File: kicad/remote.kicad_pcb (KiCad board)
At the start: 2 copper layers, 62 parts, among them J1 Conn_01x03, J10 Conn_01x03, J11 Conn_01x03, J12 Conn_01x02, J13 Conn_01x04, J14 Conn_01x04, J2 Conn_01x02, J3 Conn_01x07, J4 Conn_01x03, J5 Conn_01x03, J6 Conn_01x02, J7 Conn_01x03, J8 Conn_01x08, J9 Conn_01x08, SW1 SW_SPDT_MSM, SW10 SW_Push, SW11 SW_DP3T, SW2 SW_SPDT_MSM, SW3 SW_SPDT_MSM, SW4 SW_SPDT_MSM, SW5 SW_Push, SW6 SW_Push, SW7 SW_Push, SW8 SW_Push, SW9 SW_Push, U1 74LS165, U2 74LS165, U3 Arduino_Nano_v3.x, U4 AP1117, U5 nRF24L01+, U6 OLED_7pin_4SPI, U7 COM-09032, U8 COM-09032

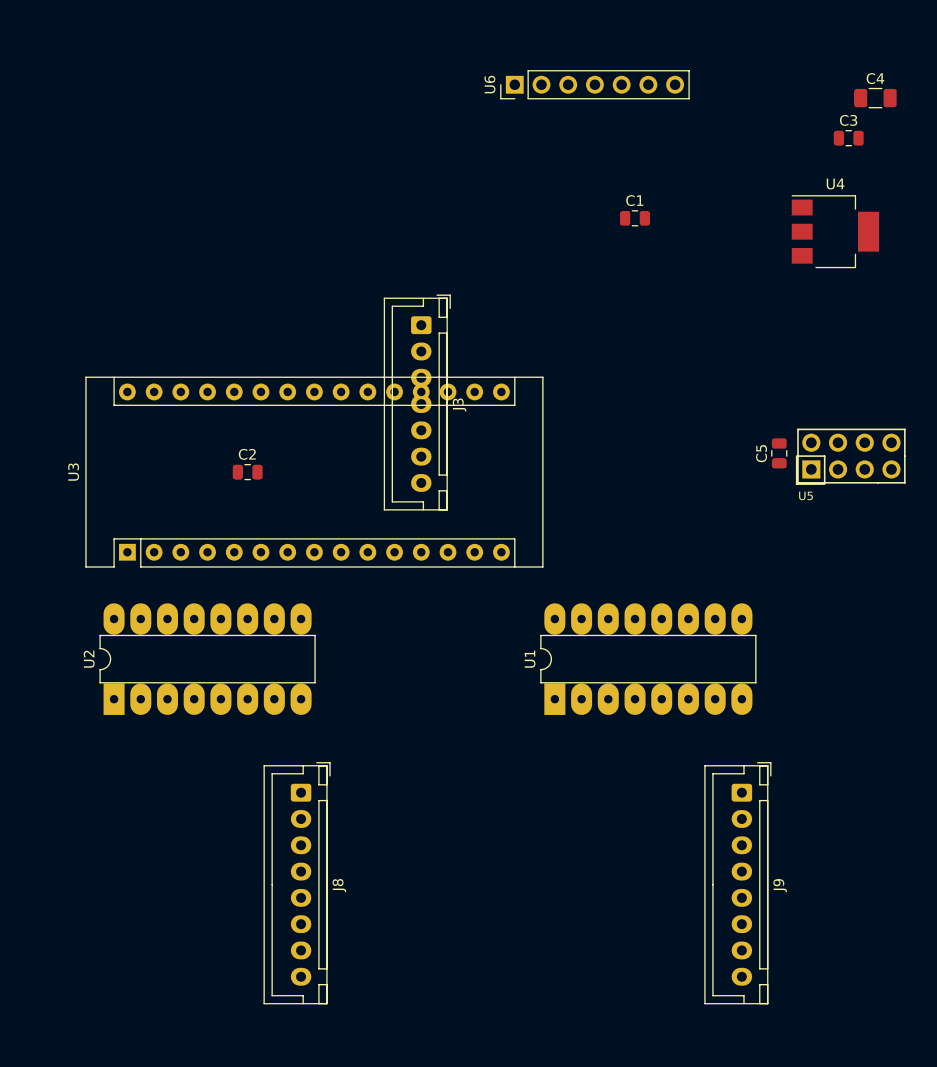
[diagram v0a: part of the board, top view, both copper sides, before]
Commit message: Work on layout.
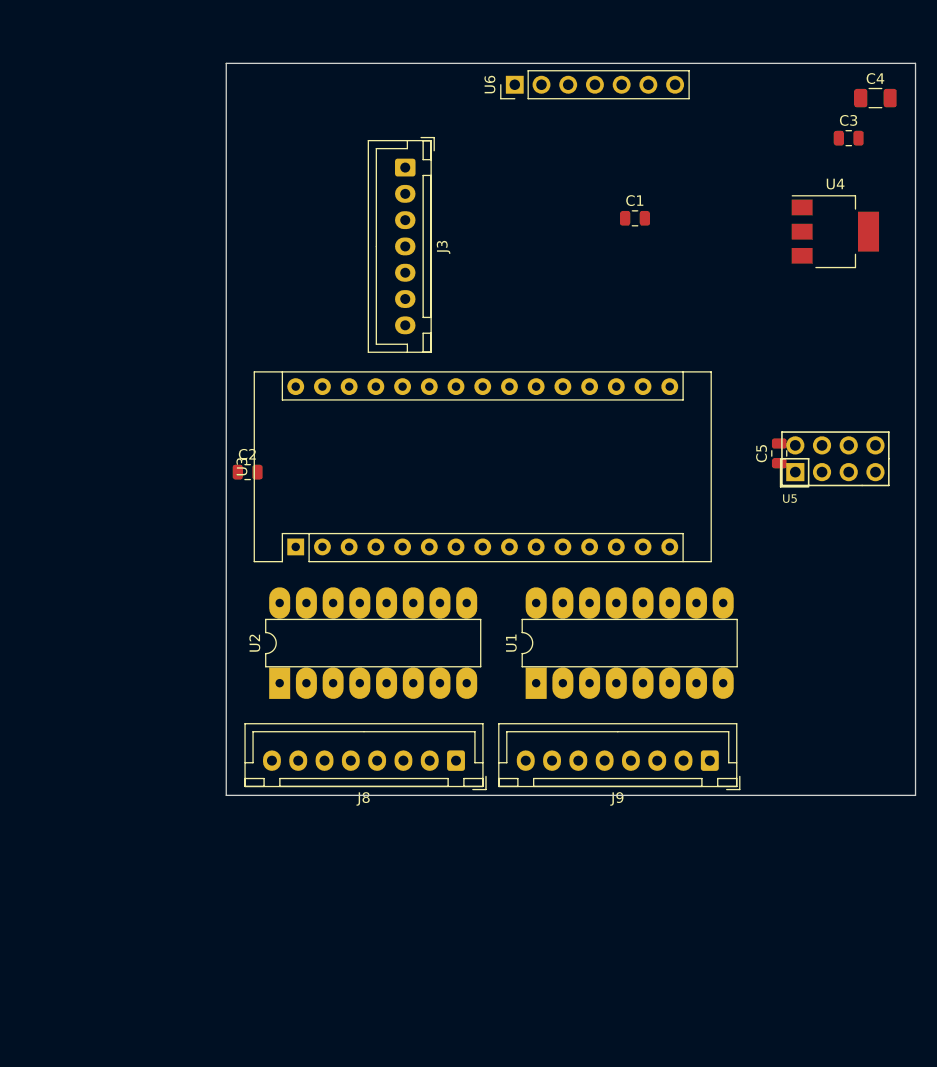
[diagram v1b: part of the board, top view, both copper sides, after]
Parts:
- moved U3 16.0 mm to (272.5, 132.8)
- moved U2 15.8 mm to (271.0, 145.8)
- moved J3 15.1 mm to (283.0, 96.8)
- moved J8 15.0 mm to (287.8, 153.2), turned to 180 degrees
- moved J9 4.31 mm to (311.9, 153.2), turned to 180 degrees
- moved U1 2.34 mm to (295.4, 145.8)
- moved U5 1.55 mm to (318.5, 127.3)
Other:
- board outline added: 65.5 x 69.6 mm
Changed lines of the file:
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@@
   (general
     (thickness 1.6)
-    (drawings 2571)
+    (drawings 2575)
     (tracks 87)
     (zones 0)
@@
   )
   (module Module:Arduino_Nano (layer F.Cu)
-    (at 256.54 133.35 90)
+    (at 272.542 132.842 90)
     (descr "Arduino Nano, http://www.mouser.com/pdfdocs/Gravitech_Arduino_Nano3_0.pdf")
     (tags "Arduino Nano")
@@
   )
   (module Remote:nRF24L01 (layer F.Cu)
-    (at 320.04 127 180)
+    (at 318.516 127.254 180)
     (descr NRF24L01)
     (tags "nRF 24 NRF24L01 NRF24L01+")
@@
   )
   (module Milling:DIP-16_W7.62mm_Milling (layer F.Cu)
-    (at 297.18 147.32 90)
+    (at 295.402 145.796 90)
     (descr "16-lead though-hole mounted DIP package, row spacing 7.62 mm (300 mils), LongPads")
     (tags "THT DIP DIL PDIP 2.54mm 7.62mm 300mil LongPads")
@@
   )
   (module Milling:DIP-16_W7.62mm_Milling (layer F.Cu)
-    (at 255.27 147.32 90)
+    (at 271.018 145.796 90)
     (descr "16-lead though-hole mounted DIP package, row spacing 7.62 mm (300 mils), LongPads")
     (tags "THT DIP DIL PDIP 2.54mm 7.62mm 300mil LongPads")
@@
   )
   (module Connector_JST:JST_XH_B07B-XH-A_1x07_P2.50mm_Vertical (layer F.Cu)
-    (at 284.48 111.76 270)
+    (at 282.956 96.774 270)
     (descr "JST XH series connector, B07B-XH-A (http://www.jst-mfg.com/product/pdf/eng/eXH.pdf), generated with kicad-footprint-generator")
     (tags "connector JST XH side entry")
@@
   )
   (module Connector_JST:JST_XH_B08B-XH-A_1x08_P2.50mm_Vertical (layer F.Cu)
-    (at 273.05 156.21 270)
+    (at 287.782 153.162 180)
     (descr "JST XH series connector, B08B-XH-A (http://www.jst-mfg.com/product/pdf/eng/eXH.pdf), generated with kicad-footprint-generator")
     (tags "connector JST XH side entry")
-    (fp_text reference J8 (at 8.75 -3.55 90) (layer F.SilkS)
+    (fp_text reference J8 (at 8.75 -3.55) (layer F.SilkS)
       (effects (font (size 1 1) (thickness 0.15)))
     )
-    (fp_text value Conn_01x08 (at 8.75 4.6 90) (layer F.Fab)
+    (fp_text value Conn_01x08 (at 8.75 4.6) (layer F.Fab)
       (effects (font (size 1 1) (thickness 0.15)))
     )
@@
     (fp_line (start -1.6 -2.75) (end -2.85 -2.75) (layer F.SilkS) (width 0.12))
     (fp_line (start -2.85 -2.75) (end -2.85 -1.5) (layer F.SilkS) (width 0.12))
-    (fp_text user %R (at 8.75 2.7 90) (layer F.Fab)
+    (fp_text user %R (at 8.75 2.7) (layer F.Fab)
       (effects (font (size 1 1) (thickness 0.15)))
     )
-    (pad 1 thru_hole roundrect (at 0 0 270) (size 1.7 1.95) (drill 0.95) (layers *.Cu *.Mask) (roundrect_rratio 0.147059)
+    (pad 1 thru_hole roundrect (at 0 0 180) (size 1.7 1.95) (drill 0.95) (layers *.Cu *.Mask) (roundrect_rratio 0.147059)
       (net 48 "Net-(J8-Pad1)"))
-    (pad 2 thru_hole oval (at 2.5 0 270) (size 1.7 1.95) (drill 0.95) (layers *.Cu *.Mask)
+    (pad 2 thru_hole oval (at 2.5 0 180) (size 1.7 1.95) (drill 0.95) (layers *.Cu *.Mask)
       (net 49 "Net-(J8-Pad2)"))
-    (pad 3 thru_hole oval (at 5 0 270) (size 1.7 1.95) (drill 0.95) (layers *.Cu *.Mask)
+    (pad 3 thru_hole oval (at 5 0 180) (size 1.7 1.95) (drill 0.95) (layers *.Cu *.Mask)
       (net 50 "Net-(J8-Pad3)"))
-    (pad 4 thru_hole oval (at 7.5 0 270) (size 1.7 1.95) (drill 0.95) (layers *.Cu *.Mask)
+    (pad 4 thru_hole oval (at 7.5 0 180) (size 1.7 1.95) (drill 0.95) (layers *.Cu *.Mask)
       (net 51 "Net-(J8-Pad4)"))
-    (pad 5 thru_hole oval (at 10 0 270) (size 1.7 1.95) (drill 0.95) (layers *.Cu *.Mask)
+    (pad 5 thru_hole oval (at 10 0 180) (size 1.7 1.95) (drill 0.95) (layers *.Cu *.Mask)
       (net 52 "Net-(J8-Pad5)"))
-    (pad 6 thru_hole oval (at 12.5 0 270) (size 1.7 1.95) (drill 0.95) (layers *.Cu *.Mask)
+    (pad 6 thru_hole oval (at 12.5 0 180) (size 1.7 1.95) (drill 0.95) (layers *.Cu *.Mask)
       (net 53 "Net-(J8-Pad6)"))
-    (pad 7 thru_hole oval (at 15 0 270) (size 1.7 1.95) (drill 0.95) (layers *.Cu *.Mask)
+    (pad 7 thru_hole oval (at 15 0 180) (size 1.7 1.95) (drill 0.95) (layers *.Cu *.Mask)
       (net 54 "Net-(J8-Pad7)"))
-    (pad 8 thru_hole oval (at 17.5 0 270) (size 1.7 1.95) (drill 0.95) (layers *.Cu *.Mask)
+    (pad 8 thru_hole oval (at 17.5 0 180) (size 1.7 1.95) (drill 0.95) (layers *.Cu *.Mask)
       (net 55 "Net-(J8-Pad8)"))
     (model ${KISYS3DMOD}/Connector_JST.3dshapes/JST_XH_B08B-XH-A_1x08_P2.50mm_Vertical.wrl
@@
   )
   (module Connector_JST:JST_XH_B08B-XH-A_1x08_P2.50mm_Vertical (layer F.Cu)
-    (at 314.96 156.21 270)
+    (at 311.912 153.162 180)
     (descr "JST XH series connector, B08B-XH-A (http://www.jst-mfg.com/product/pdf/eng/eXH.pdf), generated with kicad-footprint-generator")
     (tags "connector JST XH side entry")
-    (fp_text reference J9 (at 8.75 -3.55 90) (layer F.SilkS)
+    (fp_text reference J9 (at 8.75 -3.55) (layer F.SilkS)
       (effects (font (size 1 1) (thickness 0.15)))
     )
-    (fp_text value Conn_01x08 (at 8.75 4.6 90) (layer F.Fab)
+    (fp_text value Conn_01x08 (at 8.75 4.6) (layer F.Fab)
       (effects (font (size 1 1) (thickness 0.15)))
     )
-    (fp_text user %R (at 8.75 2.7 90) (layer F.Fab)
+    (fp_text user %R (at 8.75 2.7) (layer F.Fab)
       (effects (font (size 1 1) (thickness 0.15)))
     )
@@
     (fp_line (start -2.45 3.4) (end 19.95 3.4) (layer F.Fab) (width 0.1))
     (fp_line (start -2.45 -2.35) (end -2.45 3.4) (layer F.Fab) (width 0.1))
-    (pad 8 thru_hole oval (at 17.5 0 270) (size 1.7 1.95) (drill 0.95) (layers *.Cu *.Mask)
+    (pad 8 thru_hole oval (at 17.5 0 180) (size 1.7 1.95) (drill 0.95) (layers *.Cu *.Mask)
       (net 63 "Net-(J9-Pad8)"))
-    (pad 7 thru_hole oval (at 15 0 270) (size 1.7 1.95) (drill 0.95) (layers *.Cu *.Mask)
+    (pad 7 thru_hole oval (at 15 0 180) (size 1.7 1.95) (drill 0.95) (layers *.Cu *.Mask)
       (net 62 "Net-(J9-Pad7)"))
-    (pad 6 thru_hole oval (at 12.5 0 270) (size 1.7 1.95) (drill 0.95) (layers *.Cu *.Mask)
+    (pad 6 thru_hole oval (at 12.5 0 180) (size 1.7 1.95) (drill 0.95) (layers *.Cu *.Mask)
       (net 61 "Net-(J9-Pad6)"))
-    (pad 5 thru_hole oval (at 10 0 270) (size 1.7 1.95) (drill 0.95) (layers *.Cu *.Mask)
+    (pad 5 thru_hole oval (at 10 0 180) (size 1.7 1.95) (drill 0.95) (layers *.Cu *.Mask)
       (net 60 "Net-(J9-Pad5)"))
-    (pad 4 thru_hole oval (at 7.5 0 270) (size 1.7 1.95) (drill 0.95) (layers *.Cu *.Mask)
+    (pad 4 thru_hole oval (at 7.5 0 180) (size 1.7 1.95) (drill 0.95) (layers *.Cu *.Mask)
       (net 59 "Net-(J9-Pad4)"))
-    (pad 3 thru_hole oval (at 5 0 270) (size 1.7 1.95) (drill 0.95) (layers *.Cu *.Mask)
+    (pad 3 thru_hole oval (at 5 0 180) (size 1.7 1.95) (drill 0.95) (layers *.Cu *.Mask)
       (net 58 "Net-(J9-Pad3)"))
-    (pad 2 thru_hole oval (at 2.5 0 270) (size 1.7 1.95) (drill 0.95) (layers *.Cu *.Mask)
+    (pad 2 thru_hole oval (at 2.5 0 180) (size 1.7 1.95) (drill 0.95) (layers *.Cu *.Mask)
       (net 57 "Net-(J9-Pad2)"))
-    (pad 1 thru_hole roundrect (at 0 0 270) (size 1.7 1.95) (drill 0.95) (layers *.Cu *.Mask) (roundrect_rratio 0.147059)
+    (pad 1 thru_hole roundrect (at 0 0 180) (size 1.7 1.95) (drill 0.95) (layers *.Cu *.Mask) (roundrect_rratio 0.147059)
       (net 56 "Net-(J9-Pad1)"))
     (model ${KISYS3DMOD}/Connector_JST.3dshapes/JST_XH_B08B-XH-A_1x08_P2.50mm_Vertical.wrl
@@
     )
   )
+  (gr_line (start 265.938 86.868) (end 331.47 86.868) (layer Edge.Cuts) (width 0.05))
+  (gr_line (start 265.938 156.464) (end 265.938 86.868) (layer Edge.Cuts) (width 0.05))
+  (gr_line (start 331.47 156.464) (end 265.938 156.464) (layer Edge.Cuts) (width 0.05))
+  (gr_line (start 331.47 86.868) (end 331.47 156.464) (layer Edge.Cuts) (width 0.05))
   (gr_line (start 39.59643 266.181498) (end 42.406598 267.825204) (layer Dwgs.User) (width 0.264583))
   (gr_line (start 170.554134 138.596191) (end 170.49375 138.672657) (layer Dwgs.User) (width 0.264583))
